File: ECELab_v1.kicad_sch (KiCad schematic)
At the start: 0 parts

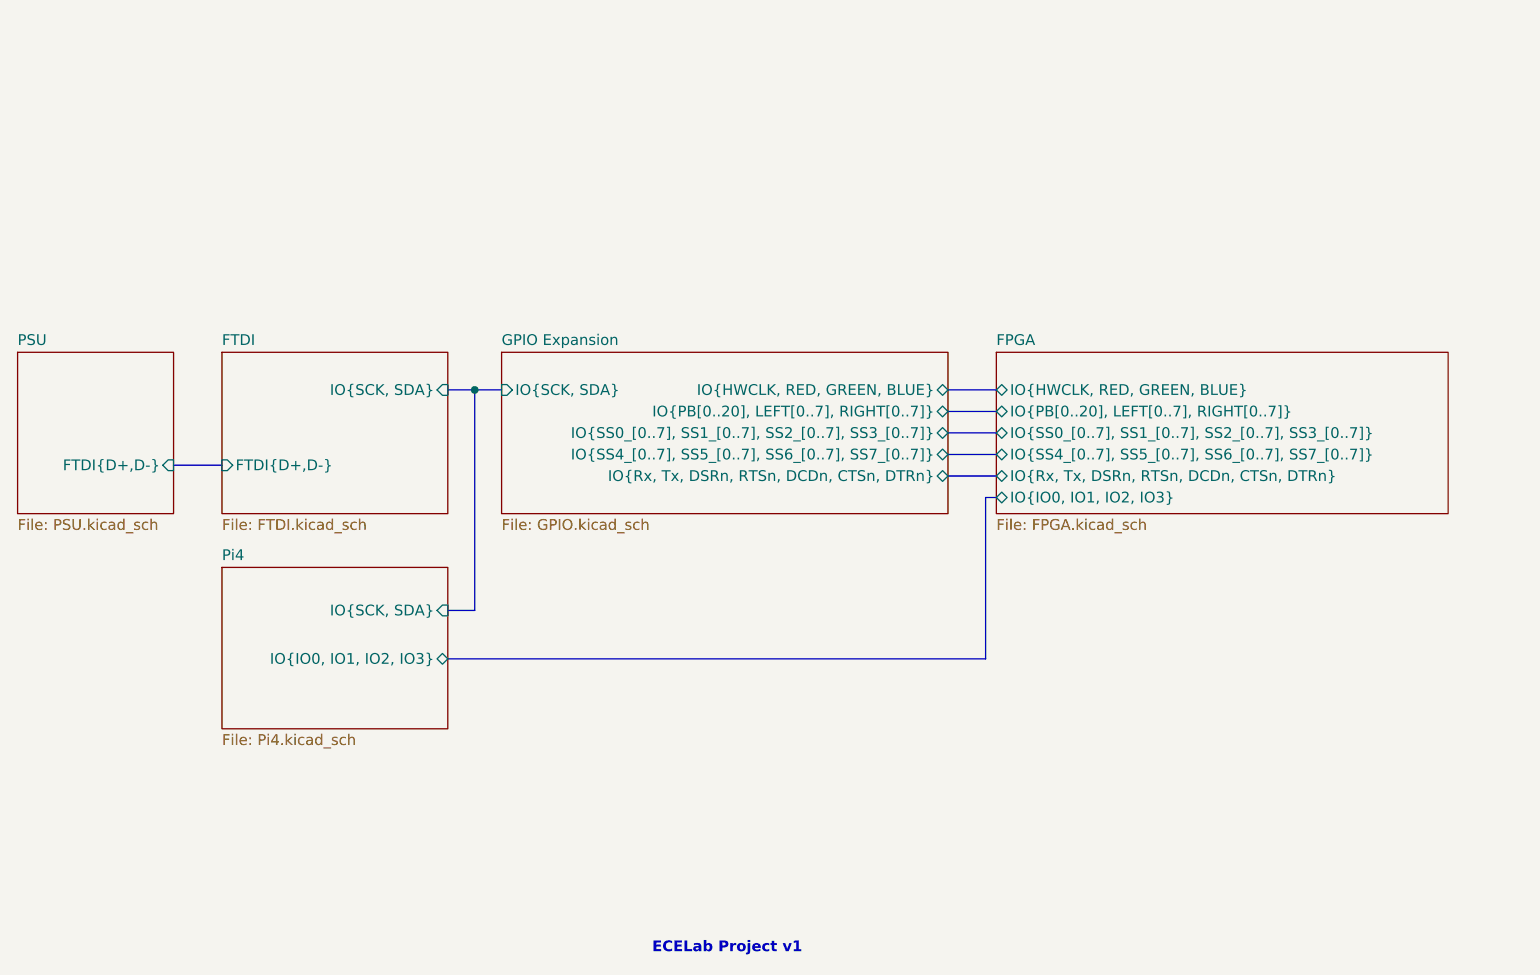
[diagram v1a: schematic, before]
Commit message: Update 2nd iteration
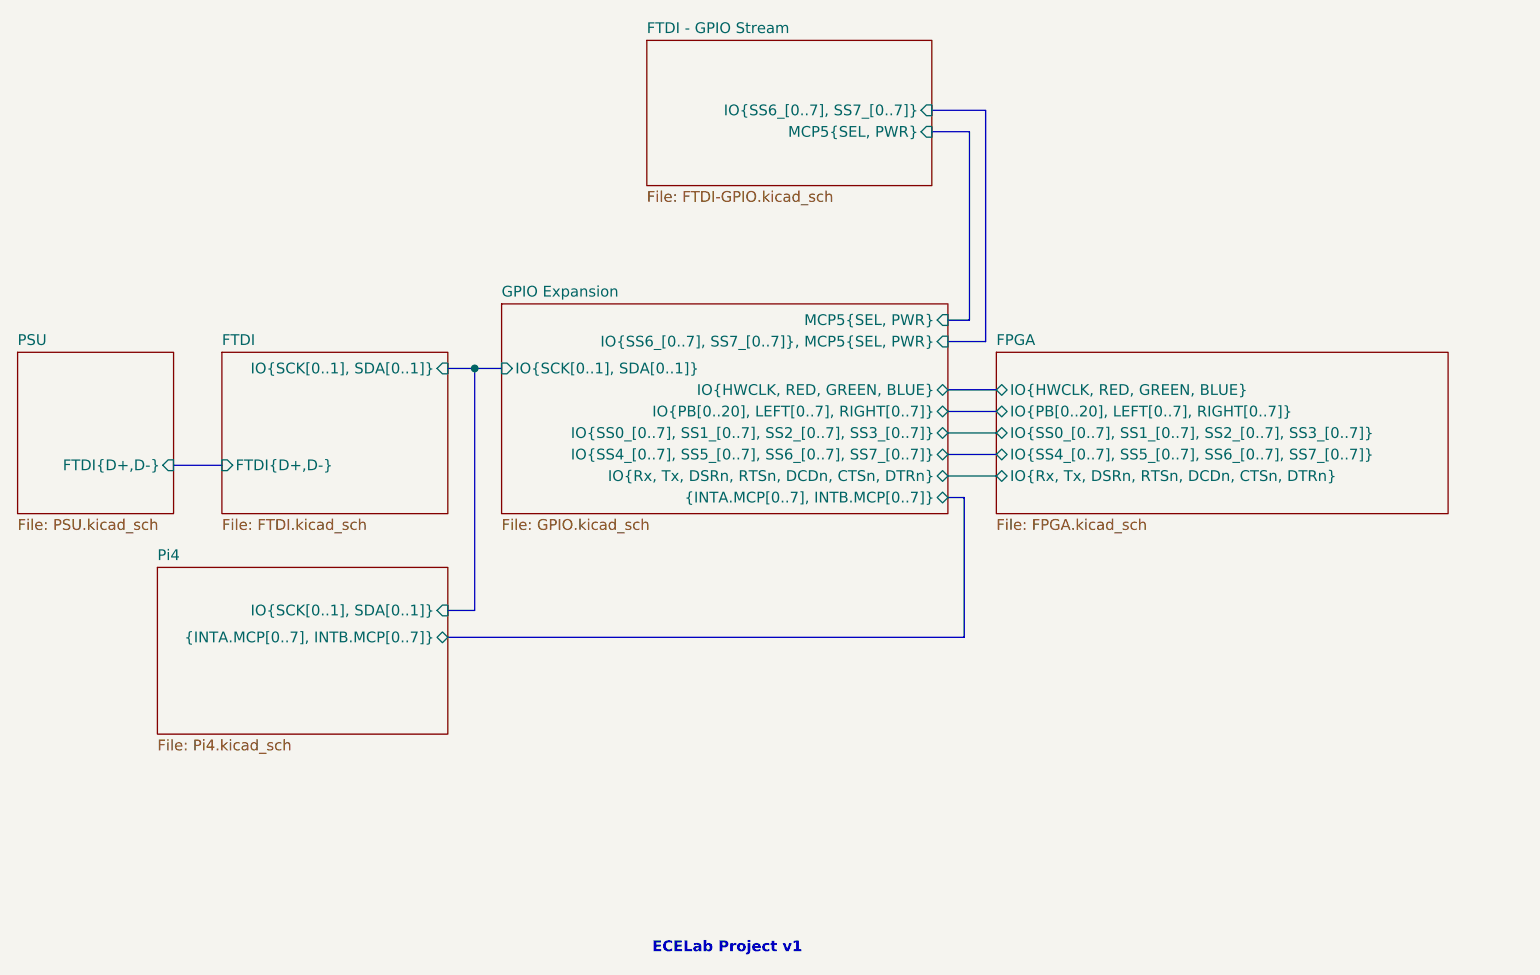
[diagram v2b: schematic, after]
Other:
- added sheet FTDI - GPIO Stream (FTDI-GPIO.kicad_sch)
- sheet FPGA ports: added none; removed IO{IO0, IO1, IO2, IO3}
- sheet FTDI ports: added IO{SCK[0..1], SDA[0..1]}; removed IO{SCK, SDA}
- sheet GPIO Expansion ports: added IO{SCK[0..1], SDA[0..1]}, IO{SS6_[0..7], SS7_[0..7]}, MCP5{SEL, PWR}, MCP5{SEL, PWR}, {INTA.MCP[0..7], INTB.MCP[0..7]}; removed IO{SCK, SDA}
- sheet Pi4 ports: added IO{SCK[0..1], SDA[0..1]}, {INTA.MCP[0..7], INTB.MCP[0..7]}; removed IO{IO0, IO1, IO2, IO3}, IO{SCK, SDA}
